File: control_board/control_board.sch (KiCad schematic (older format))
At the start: 38 parts, among them J1 Conn_01x08_Male, K1 G5Q-1A, Q1 Q_NPN_BEC, U1 MC78M05_TO252, U2 TSR_1-24120, U3 74LS02, U4 74LS02, U5 Conn_01x08_Male

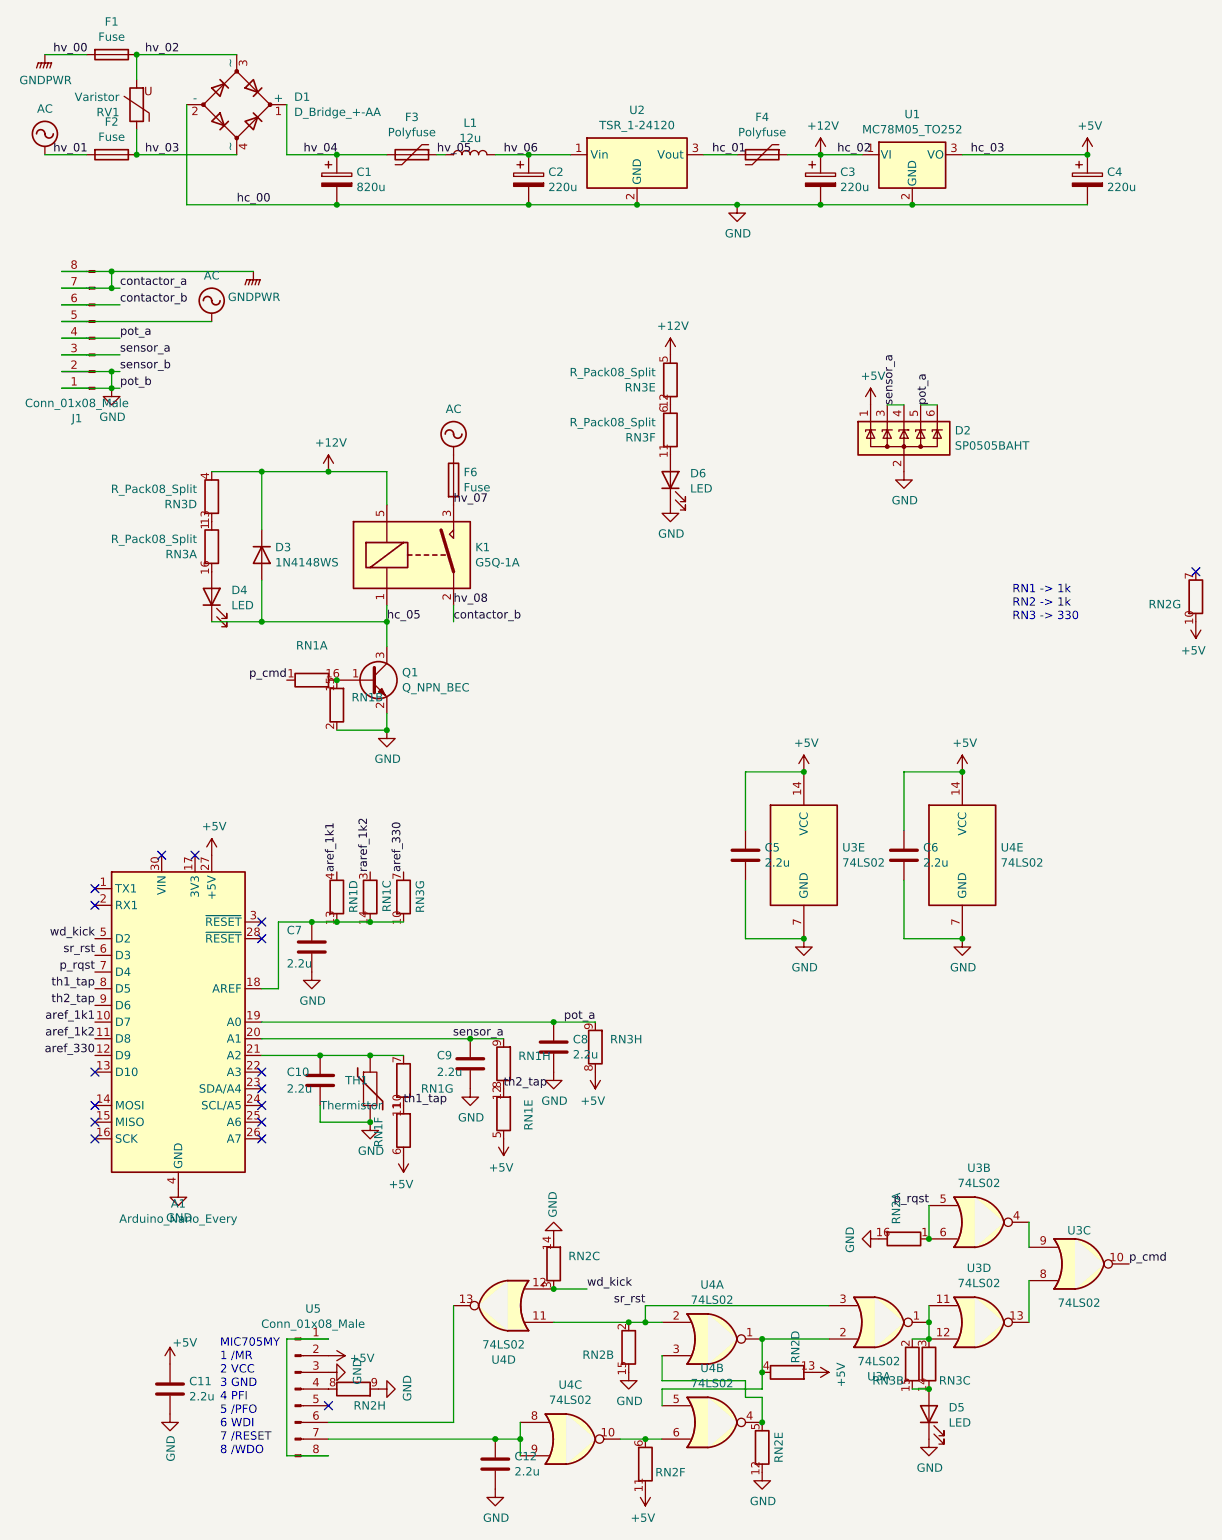
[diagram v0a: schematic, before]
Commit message: Draft logic layout
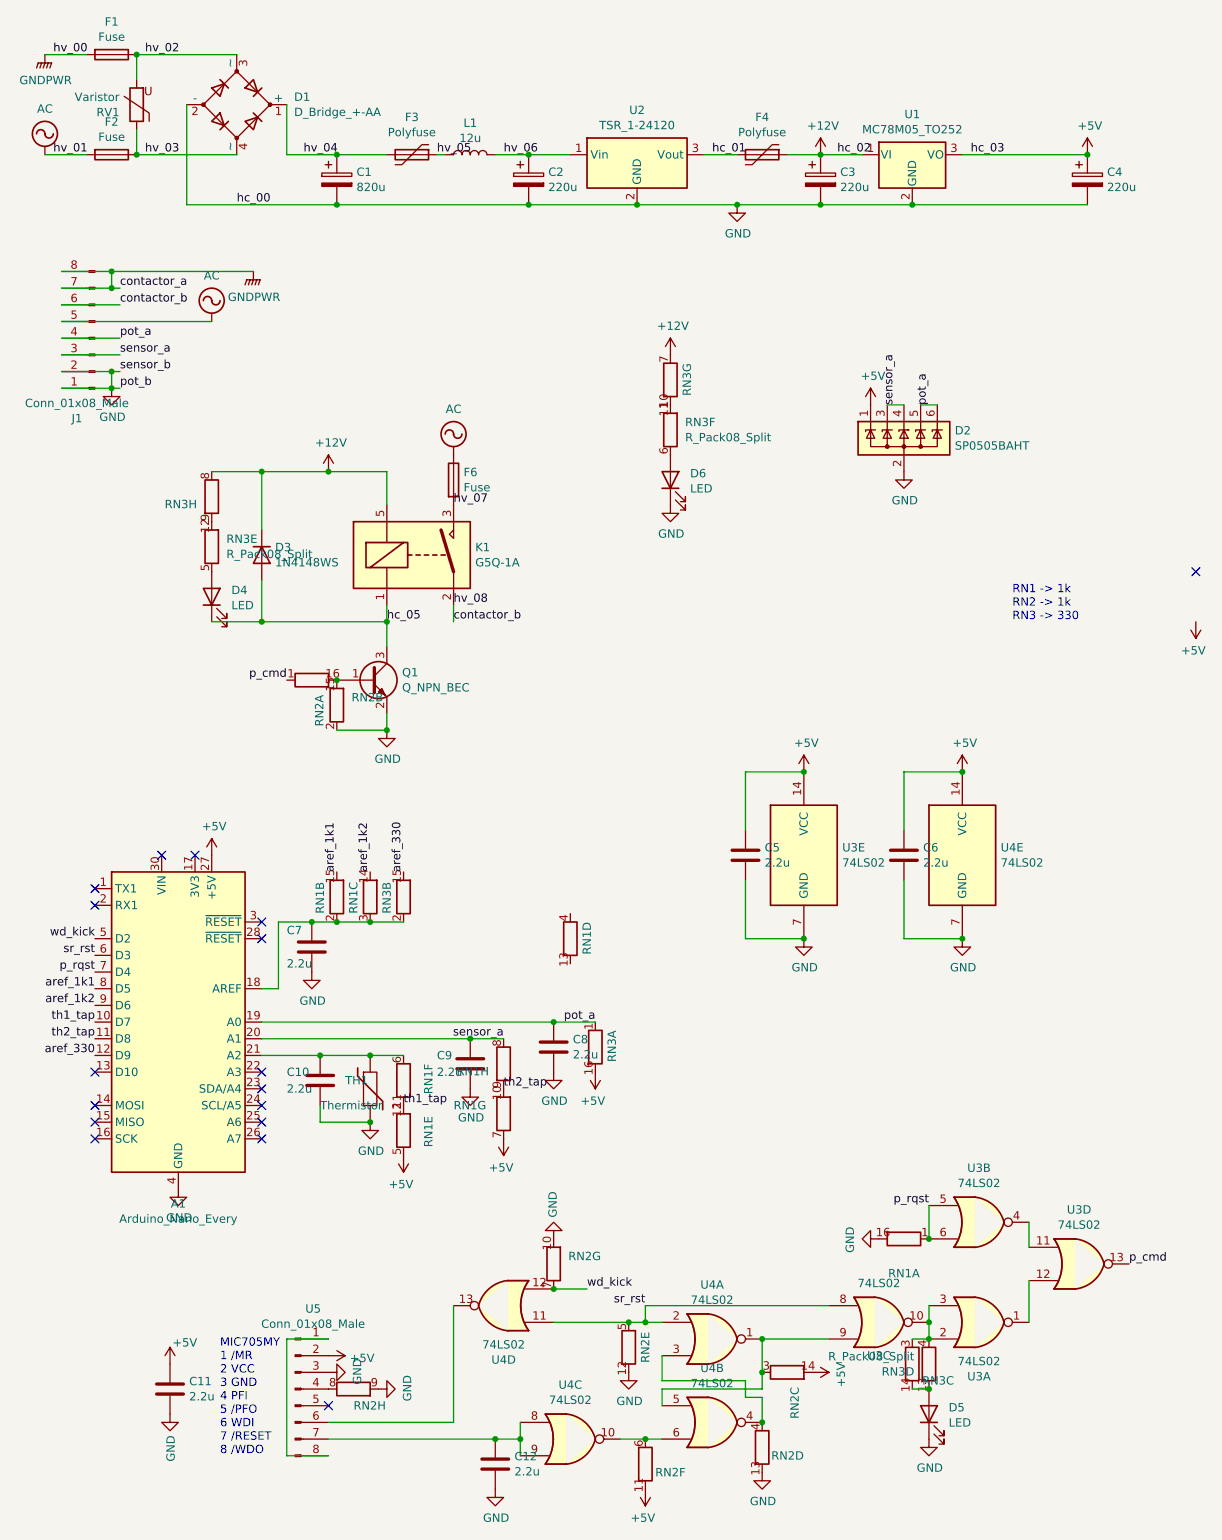
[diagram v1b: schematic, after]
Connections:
- net +12V: now also RN3.7 (R7.1), RN3.8 (R8.1); no longer RN3.4 (R4.1), RN3.5 (R5.1)
- net +5V: now also RN1.7 (R7.1), RN2.14 (R3.2), RN3.16 (R1.2); no longer RN1.6 (R6.1), RN2.10 (R7.2), RN2.13 (R4.2), RN3.8 (R8.1)
- net GND: now also RN1.16 (R1.2), RN2.10 (R7.2), RN2.13 (R4.2), RN2.2 (R2.1); no longer RN1.2 (R2.1), RN2.14 (R3.2), RN2.15 (R2.2), RN2.16 (R1.2)
- net aref_1k1: now also A1.8 (D5), RN1.15 (R2.2); no longer A1.10 (D7), RN1.4 (R4.1)
- net aref_1k2: now also A1.9 (D6), RN1.14 (R3.2); no longer A1.11 (D8)
- net aref_330: now also RN3.15 (R2.2); no longer RN3.7 (R7.1)
- net p_cmd: now also RN2.1 (R1.1), U3.13; no longer RN1.1 (R1.1), U3.10
- net p_rqst: now also RN1.1 (R1.1); no longer RN2.1 (R1.1)
- net pot_a: now also RN3.1 (R1.1); no longer RN3.9 (R8.2)
- net sensor_a: now also RN1.8 (R8.1); no longer RN1.9 (R8.2)
- net sr_rst: now also RN2.5 (R5.1), U3.8; no longer RN2.2 (R2.1), U3.3
- net th1_tap: now also A1.10 (D7), RN1.12 (R5.2); no longer A1.8 (D5), RN1.10 (R7.2)
- net th2_tap: now also A1.11 (D8), RN1.10 (R7.2), RN1.9 (R8.2); no longer A1.9 (D6), RN1.12 (R5.2), RN1.8 (R8.1)
- net wd_kick: now also RN2.7 (R7.1); no longer RN2.3 (R3.1)
- net at A1.21 (A2), C10.1, TH1.1: now also RN1.6 (R6.1); no longer RN1.7 (R7.1)
- net at D4.2 (A): now also RN3.5 (R5.1); no longer RN3.16 (R1.2)
- net at U4.1, U4.5: now also RN2.3 (R3.1), U3.9; no longer RN2.4 (R4.1), U3.2
- net at U4.3, U4.4: now also RN2.4 (R4.1); no longer RN2.5 (R5.1)
- net at D5.2 (A), RN3.14 (R3.2): now also RN3.13 (R4.2); no longer RN3.15 (R2.2)
- net at U3.4: now also U3.11; no longer U3.9
- net at D6.2 (A): now also RN3.6 (R6.1); no longer RN3.11 (R6.2)
- net at RN3.12 (R5.2): now also RN3.9 (R8.2); no longer RN3.6 (R6.1)
- net raref_1k2: no longer names the net of RN1.3 (R3.1)
- net raref_1k2: now also A1.18 (AREF), C7.1, RN1.2 (R2.1), RN3.2 (R2.1)
- new net: Q1.1 (B), RN2.15 (R2.2), RN2.16 (R1.2)
- new net: U3.1, U3.12
- new net: RN3.3 (R3.1), RN3.4 (R4.1), U3.10, U3.2, U3.3
- new net: RN3.10 (R7.2), RN3.11 (R6.2)
- now unconnected: RN1.13 (R4.2)
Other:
- moved on the sheet: RN1A, RN1B, RN1C, RN1D, RN1E, RN1F, RN1G, RN2A, RN2B, RN2C, RN2D, RN2E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
